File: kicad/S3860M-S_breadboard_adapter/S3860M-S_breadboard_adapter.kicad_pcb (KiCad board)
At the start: 2 copper layers, 26.5 x 31.6 mm, 12 parts, among them J1 SCJ368R1NUS0B00G, P1 CONN_01X12, P2 CONN_01X12, U1 S3860M-S

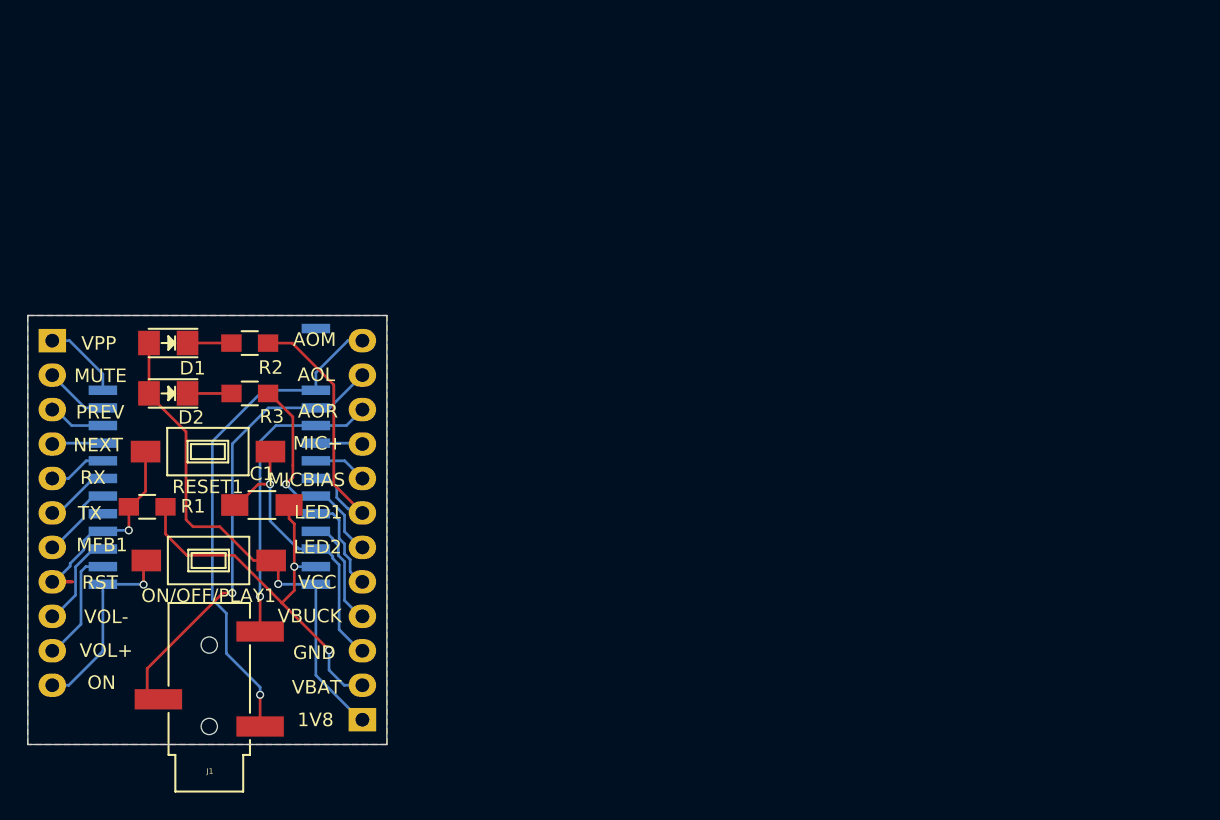
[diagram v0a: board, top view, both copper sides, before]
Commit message: version 2.0
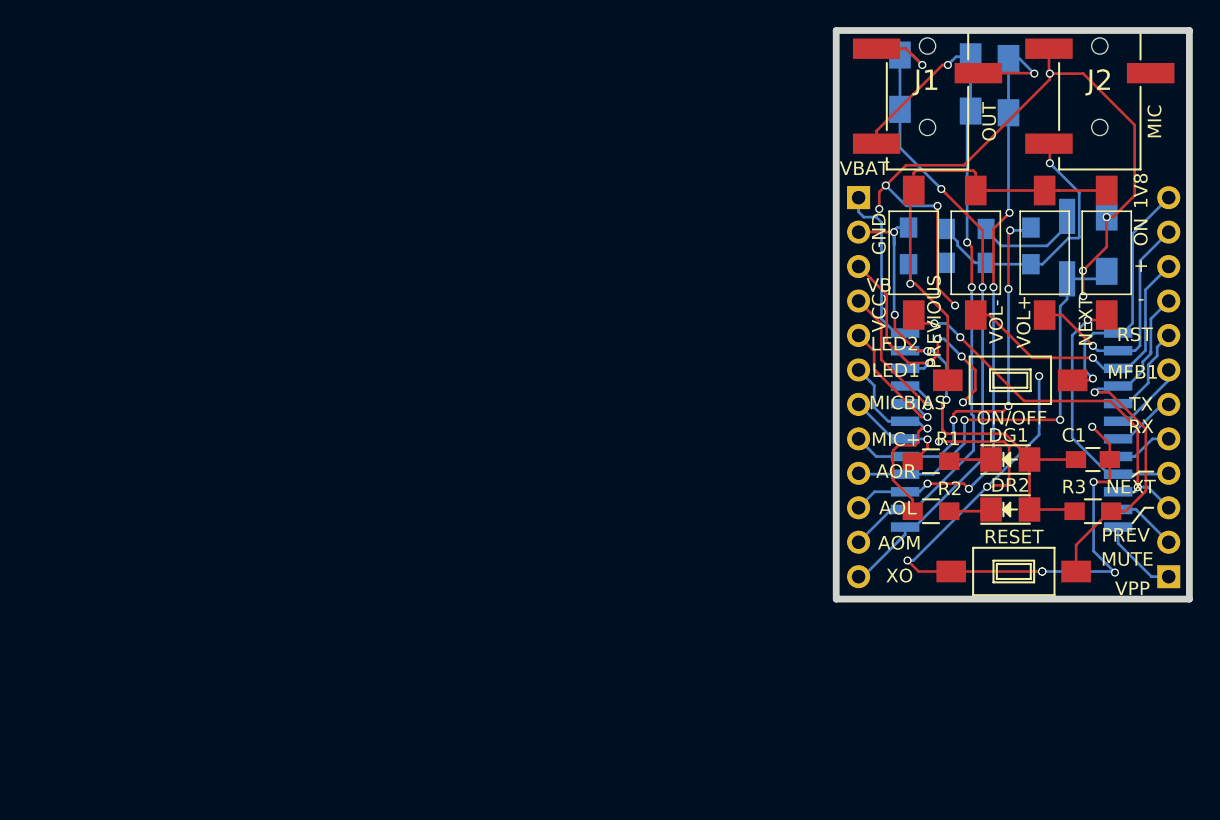
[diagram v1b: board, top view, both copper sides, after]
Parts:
- removed ON/OFF/PLAY1: ON/OFF, Buttons_Switches_SMD:SW_SPST_FSMSM
- removed the R2 at (100.9, 91.6)
- removed RESET1: 1, Buttons_Switches_SMD:SW_SPST_FSMSM
- added C2: 4u7, Capacitors_SMD.pretty:C_1206_HandSoldering, B.Cu at (164.1, 84.3)
- added C3: 2u2/6.5V, Capacitors_SMD.pretty:C_0805_HandSoldering, B.Cu at (155.2, 84.5)
- added C4: 220p/optional, Capacitors_SMD.pretty:C_0805_HandSoldering, B.Cu at (152.3, 84.5)
- added C5: 2u2, Capacitors_SMD.pretty:C_1206_HandSoldering, B.Cu at (148.8, 72.4)
- added C6: 2u2, Capacitors_SMD.pretty:C_1206_HandSoldering, B.Cu at (154.1, 72.5)
- added C7: 2u2, Capacitors_SMD.pretty:C_1206_HandSoldering, B.Cu at (156.8, 72.6)
- added J2: MIC, jacks:3.5mm_stereo_jack_PJ320B, F.Cu at (163.6, 69.7)
- added L1: 15n, Choke_SMD.pretty:Choke_SMD_1206_Handsoldering, B.Cu at (161.2, 84.6)
- added R1: 470, Resistors_SMD:R_0805_HandSoldering, F.Cu at (151.1, 100.3)
- added R4: 2k2, Resistors_SMD:R_0805_HandSoldering, B.Cu at (158.5, 84.5)
- added R5: 2k, Resistors_SMD:R_0805_HandSoldering, B.Cu at (149.5, 84.5)
- added SW1: PREVIOUS, Buttons_Switches_SMD:SW_SPST_FSMSM, F.Cu at (149.9, 85.0)
- added SW2: NEXT, Buttons_Switches_SMD:SW_SPST_FSMSM, F.Cu at (164.1, 85.0)
- added SW3: VOL-, Buttons_Switches_SMD:SW_SPST_FSMSM, F.Cu at (154.4, 85.0)
- added SW4: VOL+, Buttons_Switches_SMD:SW_SPST_FSMSM, F.Cu at (159.5, 85.0)
- added SW5: ON/OFF, Buttons_Switches_SMD:SW_SPST_FSMSM, F.Cu at (157.0, 94.4)
- added SW6: RESET, Buttons_Switches_SMD:SW_SPST_FSMSM, F.Cu at (157.2, 108.5)
- C1: footprint Capacitors_SMD.pretty:C_1206_HandSoldering -> Capacitors_SMD.pretty:C_0805_HandSoldering
- DG1: renamed from D1; value LED -> GREEN
- DR2: renamed from D2; value LED -> RED
- J1: value SCJ368R1NUS0B00G -> OUT
- P1: footprint Pin_Headers:Pin_Header_Straight_1x12 -> Pin_Headers:Pin_Header_Straight_1x12_Pitch2.54mm
- P2: footprint Pin_Headers:Pin_Header_Straight_1x11 -> Pin_Headers:Pin_Header_Straight_1x12_Pitch2.54mm
- U1: footprint my_modules:XS3868 -> bluetooth:S3860M-S
- moved P2 84.1 mm to (168.7, 108.8), turned to 0 degrees
- moved J1 72.9 mm to (150.9, 69.7), turned to 0 degrees
- moved R3 69.7 mm to (163.1, 104.0), turned to 180 degrees
- moved DG1 62.7 mm to (157.0, 100.2), turned to 0 degrees
- moved DR2 62.6 mm to (157.0, 103.9), turned to 0 degrees
- moved C1 61.3 mm to (163.1, 100.2), turned to 180 degrees
- moved P1 53.1 mm to (145.8, 80.9), turned to 180 degrees
- moved R2 51.0 mm to (151.1, 104.0), turned to 180 degrees
- moved U1 48.5 mm to (149.2, 89.3), turned to 0 degrees
- renumbered R3 to R2, R1 to R3
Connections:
- net /GND renamed GND
- net Net-(J1-Pad1) renamed /AOM
- net Net-(J1-Pad2) renamed /AOL
- net Net-(P1-Pad4) renamed /VBUCK
- net Net-(P1-Pad5) renamed /VCC
- net Net-(P1-Pad6) renamed /LED2
- net Net-(P1-Pad7) renamed /LED1
- net Net-(P1-Pad8) renamed /MICBIAS
- net Net-(P1-Pad9) renamed /MIC+
- net Net-(P2-Pad1) renamed /VPP
- net Net-(P2-Pad2) renamed /MUTE
- net Net-(P2-Pad3) renamed /PREVIOUS
- net Net-(P2-Pad4) renamed /NEXT
- net Net-(P2-Pad5) renamed /UART_RX
- net Net-(P2-Pad6) renamed /UART_TX
- net Net-(P2-Pad7) renamed /MFB1
- C1 pad 2: Net-(C1-Pad2) -> /VBAT
- DG1 pad 2: Net-(D1-Pad2) -> /VBAT
- DR2 pad 2: Net-(D1-Pad2) -> /VBAT
- P1 pad 1: Net-(D1-Pad2) -> /1V8
- P1 pad 10: Net-(J1-Pad5) -> /AOR
- P1 pad 2: Net-(C1-Pad2) -> /VBAT
- P2 pad 10: Net-(P2-Pad10) -> /VOL-
- P2 pad 11: Net-(ON/OFF/PLAY1-Pad2) -> /VOL+
- P2 pad 9: Net-(P2-Pad9) -> /RESET
- R3 pad 1: Net-(P2-Pad8) -> /RESET
- R3 pad 2: Net-(C1-Pad2) -> /VBAT
- U1 pad 1: (no net) -> Net-(U1-Pad1)
- U1 pad 12: Net-(C1-Pad2) -> /VBAT
- U1 pad 13: Net-(D1-Pad2) -> /1V8
- U1 pad 14: Net-(ON/OFF/PLAY1-Pad2) -> /ONKEY
- U1 pad 15: Net-(P2-Pad10) -> /VOL+
- U1 pad 16: Net-(P2-Pad9) -> /VOL-
- U1 pad 17: Net-(P2-Pad8) -> /RESET
- U1 pad 18: (no net) -> Net-(P2-Pad8)
- U1 pad 4: Net-(J1-Pad5) -> /AOR
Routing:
- net GND: track 22.6 -> 131.3 mm, vias 1 -> 21
- net /AOR: track 0.00 -> 48.5 mm, vias 0 -> 5
- net /VBAT: track 0.00 -> 42.5 mm, vias 0 -> 4
- net Net-(D1-Pad2): track 39.3 -> 0.00 mm, vias 1 -> 0
- net /MIC+: track 3.46 -> 39.9 mm, vias 0 -> 2
- net Net-(R5-Pad2): track 0.00 -> 33.9 mm, vias 0 -> 1
- net Net-(C1-Pad2): track 32.3 -> 0.00 mm, vias 2 -> 0
- net /RESET: track 0.00 -> 28.5 mm, vias 0 -> 1
- net /MICBIAS: track 3.97 -> 29.0 mm, vias 0 -> 4
- net /PREVIOUS: track 4.22 -> 28.9 mm, vias 0 -> 3
- net Net-(J1-Pad5): track 22.5 -> 0.00 mm, vias 1 -> 0
- net /VOL-: track 0.00 -> 21.9 mm, vias 0 -> 1
- net Net-(C3-Pad2): track 0.00 -> 19.7 mm, vias 0 -> 1
- net /ONKEY: track 0.00 -> 19.0 mm, vias 0 -> 1
- net /VOL+: track 0.00 -> 17.5 mm, vias 0 -> 1
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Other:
- board size 26.5 x 31.6 mm -> 26 x 41.9 mm
- board text added: "+"
- board text added: "-"
- board text added: "VB"
- board text added: "XO"
- board text removed: "VBUCK"
- board text removed: "VOL+"
- board text removed: "VOL-"
